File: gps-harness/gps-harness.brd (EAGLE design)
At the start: 30.1 x 33 mm, 7 parts

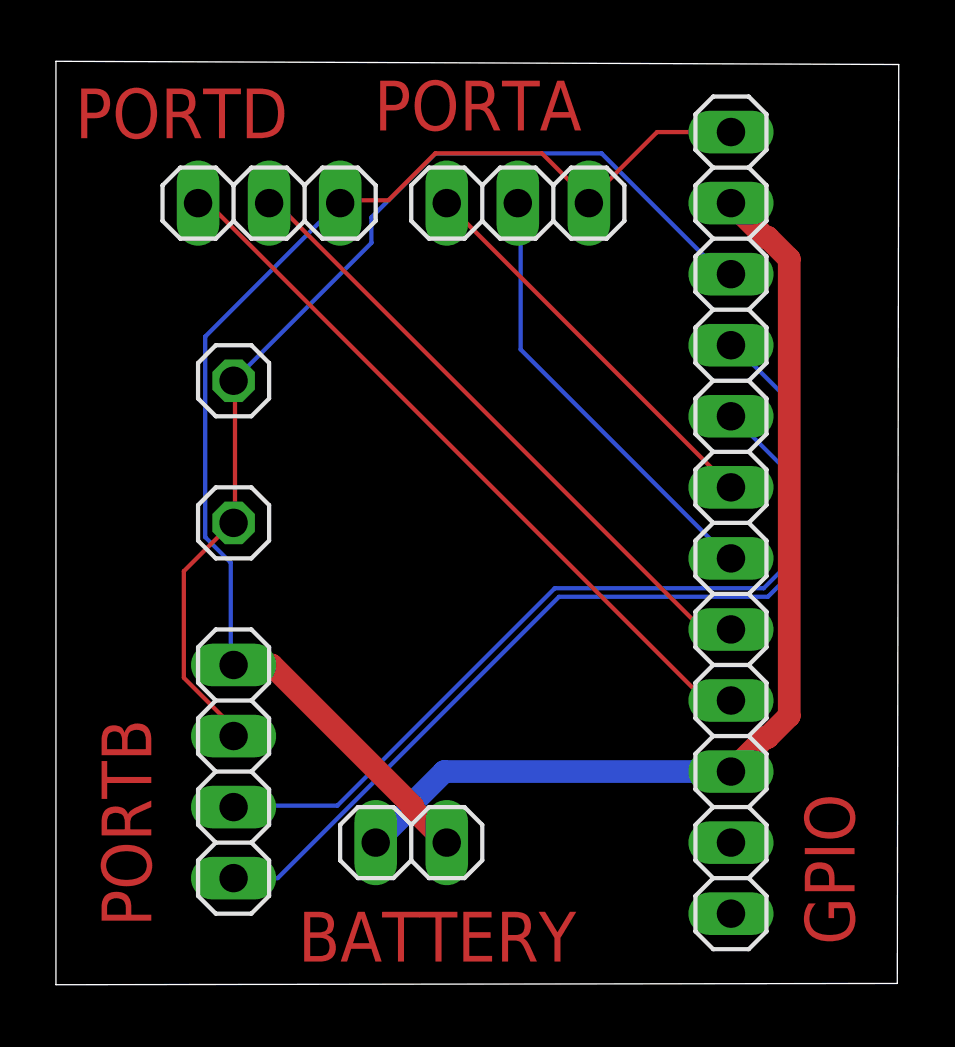
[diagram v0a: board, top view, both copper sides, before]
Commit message: Trying to choose the connector
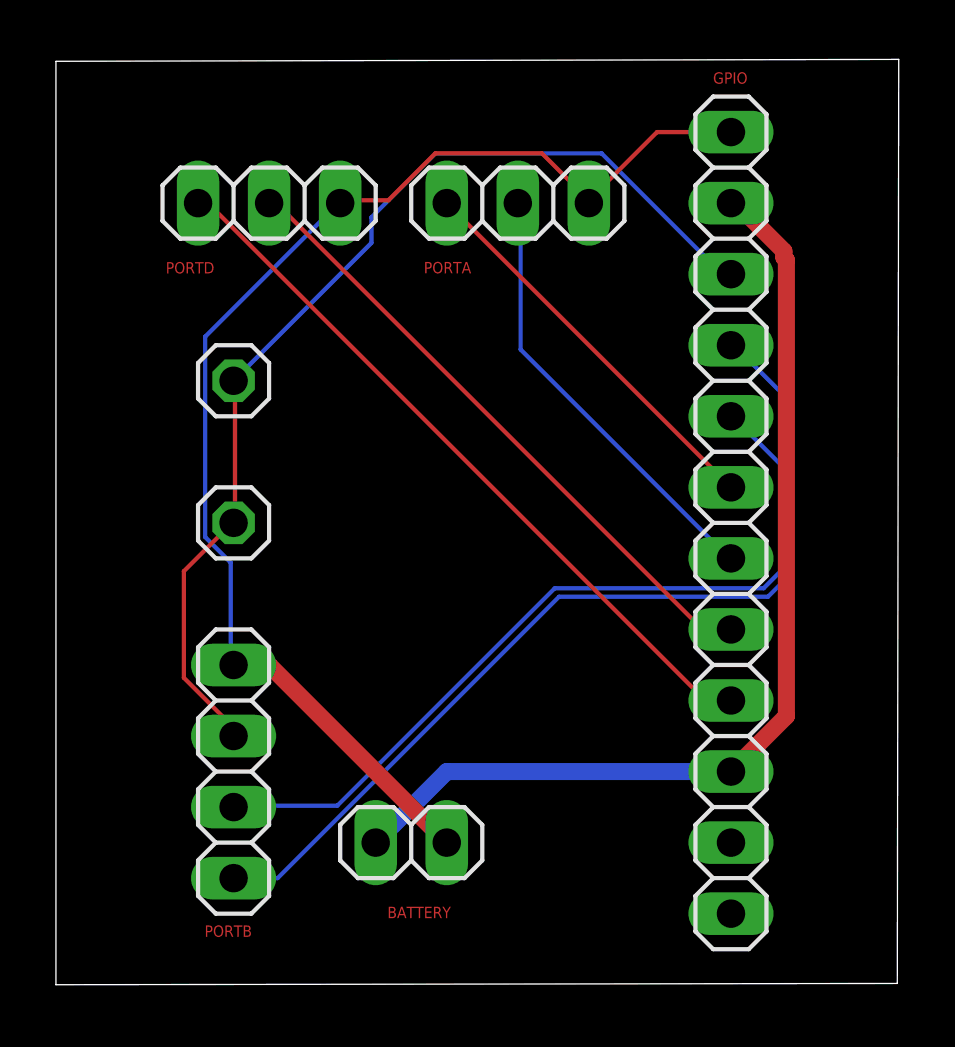
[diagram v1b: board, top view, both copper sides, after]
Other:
- board size 30.1 x 33 mm -> 30.1 x 33.1 mm
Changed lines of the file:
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@@
 <layer number="28" name="bValues" color="7" fill="1" visible="yes" active="yes"/>
 <layer number="29" name="tStop" color="7" fill="3" visible="no" active="yes"/>
-<layer number="30" name="bStop" color="7" fill="6" visible="no" active="yes"/>
+<layer number="30" name="bStop" color="7" fill="6" visible="yes" active="yes"/>
 <layer number="31" name="tCream" color="7" fill="4" visible="no" active="yes"/>
 <layer number="32" name="bCream" color="7" fill="5" visible="no" active="yes"/>
@@
 <plain>
 <wire x1="0" y1="0" x2="30.0763375" y2="0.04571875" width="0" layer="20"/>
-<wire x1="30.0763375" y1="0.04571875" x2="30.127103125" y2="32.895340625" width="0" layer="20"/>
-<wire x1="30.127103125" y1="32.895340625" x2="0" y2="33.01" width="0" layer="20"/>
+<wire x1="30.0763375" y1="0.04571875" x2="30.127103125" y2="33.078221875" width="0" layer="20"/>
+<wire x1="30.127103125" y1="33.078221875" x2="0" y2="33.01" width="0" layer="20"/>
 <wire x1="0" y1="33.01" x2="0" y2="0" width="0" layer="20"/>
-<text x="0.688340625" y="30.259021875" size="1.778" layer="1">PORTD</text>
-<text x="11.37411875" y="30.53841875" size="1.778" layer="1">PORTA</text>
-<text x="3.408678125" y="2.072640625" size="1.778" layer="1" rot="R90">PORTB</text>
-<text x="8.65631875" y="0.828040625" size="1.778" layer="1">BATTERY</text>
-<text x="28.5470625" y="1.42748125" size="1.778" layer="1" rot="R90">GPIO</text>
+<text x="3.924303125" y="25.425403125" size="0.4064" layer="1">PORTD</text>
+<text x="13.149578125" y="25.430478125" size="0.4064" layer="1">PORTA</text>
+<text x="7.00785625" y="2.1183625" size="0.4064" layer="1" rot="R180">PORTB</text>
+<text x="11.84655625" y="2.37998125" size="0.4064" layer="1">BATTERY</text>
+<text x="23.489921875" y="32.209740625" size="0.4064" layer="1">GPIO</text>
 </plain>
 <attributes>
@@
 <contactref element="BATTERY" pad="2"/>
 <wire x1="11.8872" y1="28.0416" x2="10.2108" y2="28.0416" width="0.1524" layer="1"/>
-<wire x1="13.5636" y1="29.718" x2="11.8872" y2="28.0416" width="0.1524" layer="1"/>
+<wire x1="11.8872" y1="28.0416" x2="13.5636" y2="29.718" width="0.1524" layer="1"/>
 <wire x1="17.3736" y1="29.718" x2="13.5636" y2="29.718" width="0.1524" layer="1"/>
-<wire x1="19.05" y1="28.0416" x2="17.3736" y2="29.718" width="0.1524" layer="1"/>
+<wire x1="17.3736" y1="29.718" x2="19.05" y2="28.0416" width="0.1524" layer="1"/>
 <wire x1="10.2108" y1="28.0416" x2="10.16" y2="27.94" width="0.1524" layer="1"/>
 <wire x1="21.4884" y1="30.48" x2="24.13" y2="30.48" width="0.1524" layer="1"/>
@@
 <wire x1="6.2484" y1="11.43" x2="6.35" y2="11.43" width="0.1524" layer="16"/>
 <wire x1="10.0584" y1="27.8892" x2="10.16" y2="27.94" width="0.1524" layer="16"/>
-<wire x1="13.97" y1="5.08" x2="12.7508" y2="6.2992" width="0.8128" layer="1"/>
-<wire x1="12.7508" y1="6.2992" x2="12.7508" y2="6.38909375" width="0.8128" layer="1"/>
-<wire x1="12.7508" y1="6.38909375" x2="7.70989375" y2="11.43" width="0.8128" layer="1"/>
-<wire x1="7.70989375" y1="11.43" x2="6.35" y2="11.43" width="0.8128" layer="1"/>
+<wire x1="6.35" y1="11.43" x2="7.62" y2="11.43" width="0.6096" layer="1"/>
+<wire x1="7.62" y1="11.43" x2="13.97" y2="5.08" width="0.6096" layer="1"/>
 </signal>
 <signal name="RXA">
@@
 <contactref element="GPIO" pad="2"/>
 <contactref element="GPIO" pad="10"/>
-<wire x1="24.03601875" y1="7.62" x2="24.13" y2="7.62" width="0.3048" layer="16"/>
-<wire x1="25.43909375" y1="26.7208" x2="26.2128" y2="25.94709375" width="0.8128" layer="1"/>
-<wire x1="26.2128" y1="9.61290625" x2="25.43909375" y2="8.8392" width="0.8128" layer="1"/>
-<wire x1="24.13" y1="27.94" x2="25.3492" y2="26.7208" width="0.8128" layer="1"/>
-<wire x1="25.3492" y1="26.7208" x2="25.43909375" y2="26.7208" width="0.8128" layer="1"/>
-<wire x1="25.43909375" y1="8.8392" x2="25.3492" y2="8.8392" width="0.8128" layer="1"/>
-<wire x1="25.3492" y1="8.8392" x2="24.13" y2="7.62" width="0.8128" layer="1"/>
-<wire x1="26.2128" y1="25.94709375" x2="26.2128" y2="9.61290625" width="0.8128" layer="1"/>
-<wire x1="11.43" y1="5.08" x2="12.6492" y2="6.2992" width="0.8128" layer="16"/>
-<wire x1="12.6492" y1="6.2992" x2="12.6492" y2="6.38909375" width="0.8128" layer="16"/>
-<wire x1="12.6492" y1="6.38909375" x2="13.88010625" y2="7.62" width="0.8128" layer="16"/>
-<wire x1="13.88010625" y1="7.62" x2="24.03601875" y2="7.62" width="0.8128" layer="16"/>
+<wire x1="24.03601875" y1="7.62" x2="24.107140625" y2="7.62" width="0.3048" layer="16"/>
+<wire x1="24.107140625" y1="7.62" x2="24.13" y2="7.62" width="0.3048" layer="16"/>
+<wire x1="26.1112" y1="25.9050125" x2="26.0223" y2="25.9939125" width="0.6096" layer="1"/>
+<wire x1="26.0223" y1="25.9939125" x2="26.0223" y2="26.222959375" width="0.6096" layer="1"/>
+<wire x1="24.13" y1="7.62" x2="26.1112" y2="9.6012" width="0.6096" layer="1"/>
+<wire x1="26.1112" y1="9.6012" x2="26.1112" y2="25.9050125" width="0.6096" layer="1"/>
+<wire x1="26.0223" y1="26.222959375" x2="24.305259375" y2="27.94" width="0.6096" layer="1"/>
+<wire x1="24.305259375" y1="27.94" x2="24.13" y2="27.94" width="0.6096" layer="1"/>
+<wire x1="11.43" y1="5.08" x2="13.97" y2="7.62" width="0.6096" layer="16"/>
+<wire x1="13.97" y1="7.62" x2="24.107140625" y2="7.62" width="0.6096" layer="16"/>
 </signal>
 <signal name="TXD">
